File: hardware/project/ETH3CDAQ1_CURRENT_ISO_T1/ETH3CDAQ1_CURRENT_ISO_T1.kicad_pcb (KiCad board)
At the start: 4 copper layers, 80 x 30 mm, 52 parts, among them J1 PC 5/2-G-7.62, J2 Conn_02x10_Odd_Even, U1 DG419xY, U10 74LVC1GU04DRL, U11 TXB0104PW, U2 DG211, U3 T60404-N4646-X400, U4 OPA140, U5 LT3032-15, U6 24LC08B-E/MS, U7 PCA9557PW, U8 74LVC1GU04DRL, U9 74LVC1GU04DRL

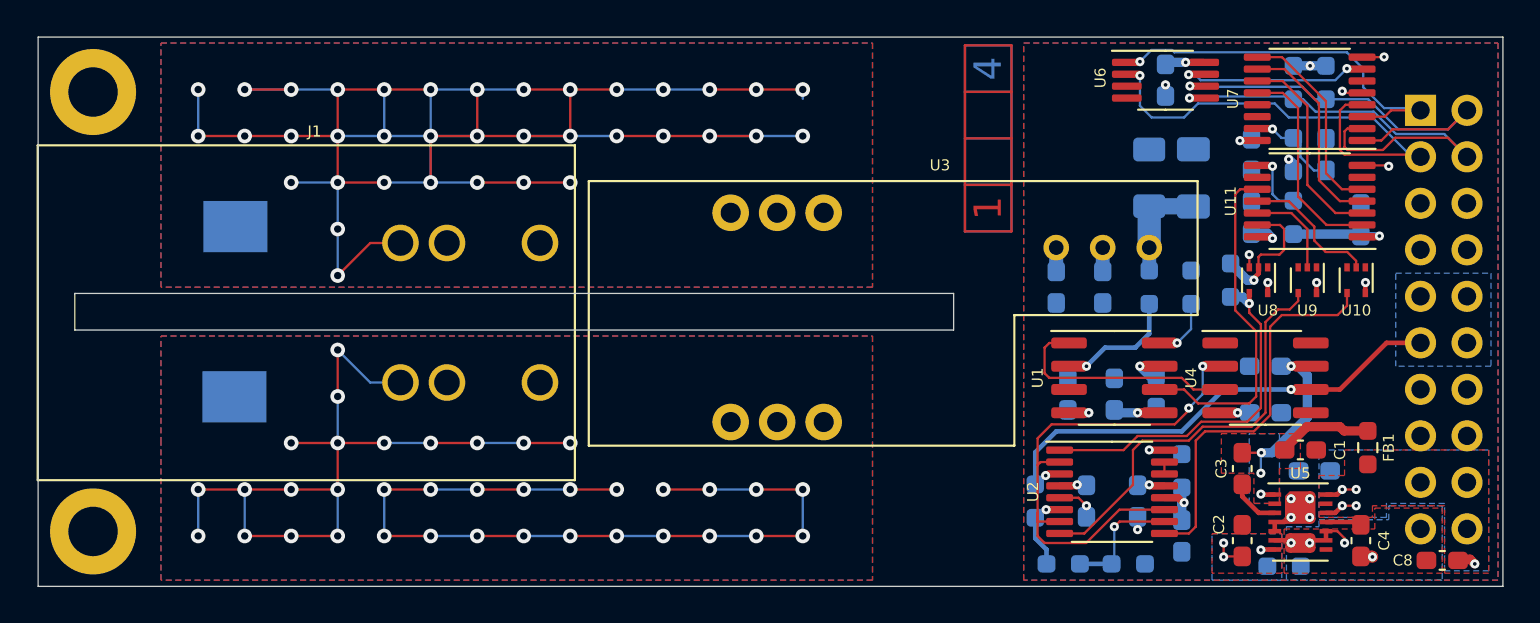
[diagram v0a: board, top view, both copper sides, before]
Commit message: PCB modifications
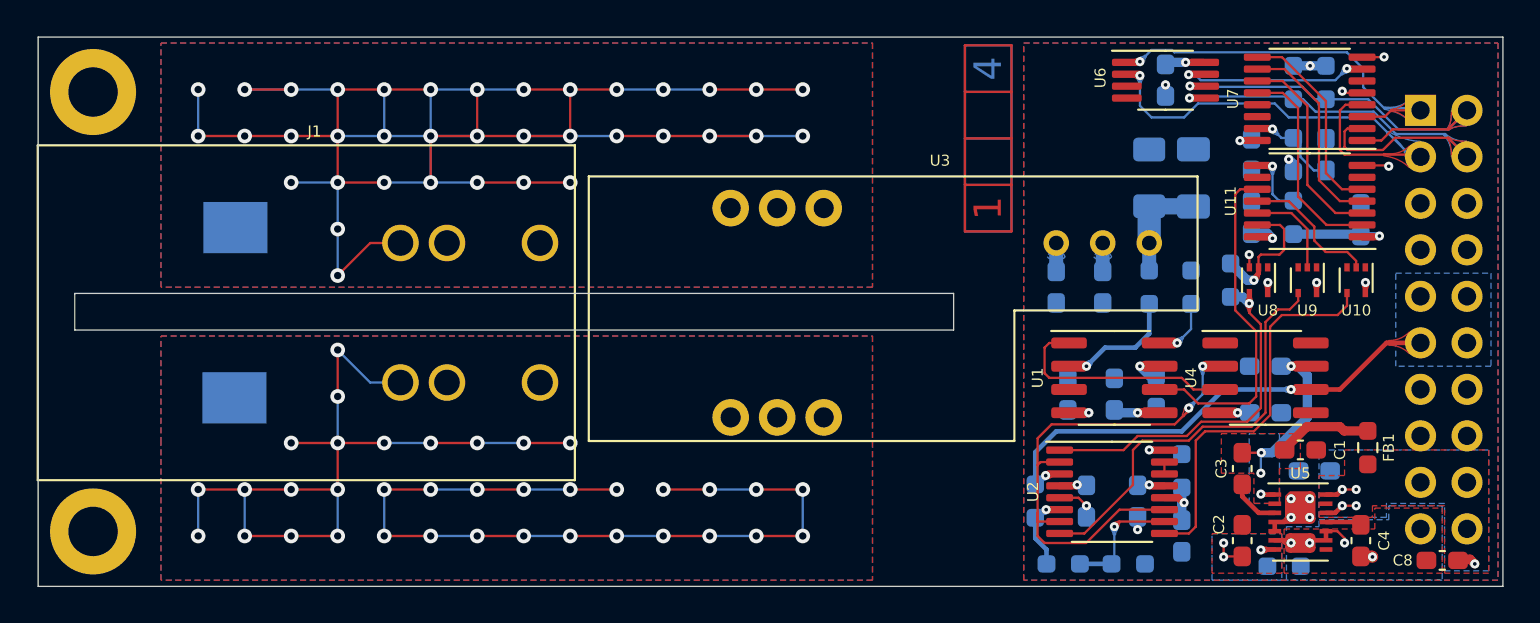
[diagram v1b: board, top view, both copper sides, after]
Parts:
- moved U3 0.25 mm to (119.3, 67.1)
- moved RV1 0.06 mm to (80.8, 67.1)
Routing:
- net Net-(J1-Pad1): track 121.8 -> 121.3 mm
